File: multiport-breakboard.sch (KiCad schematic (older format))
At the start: 6 parts, among them J1 USB_terminal, J2 USB_B_Micro, J3 soldier_pads, J4 MULT_terminal, SW1 SW_SPDT_MSM

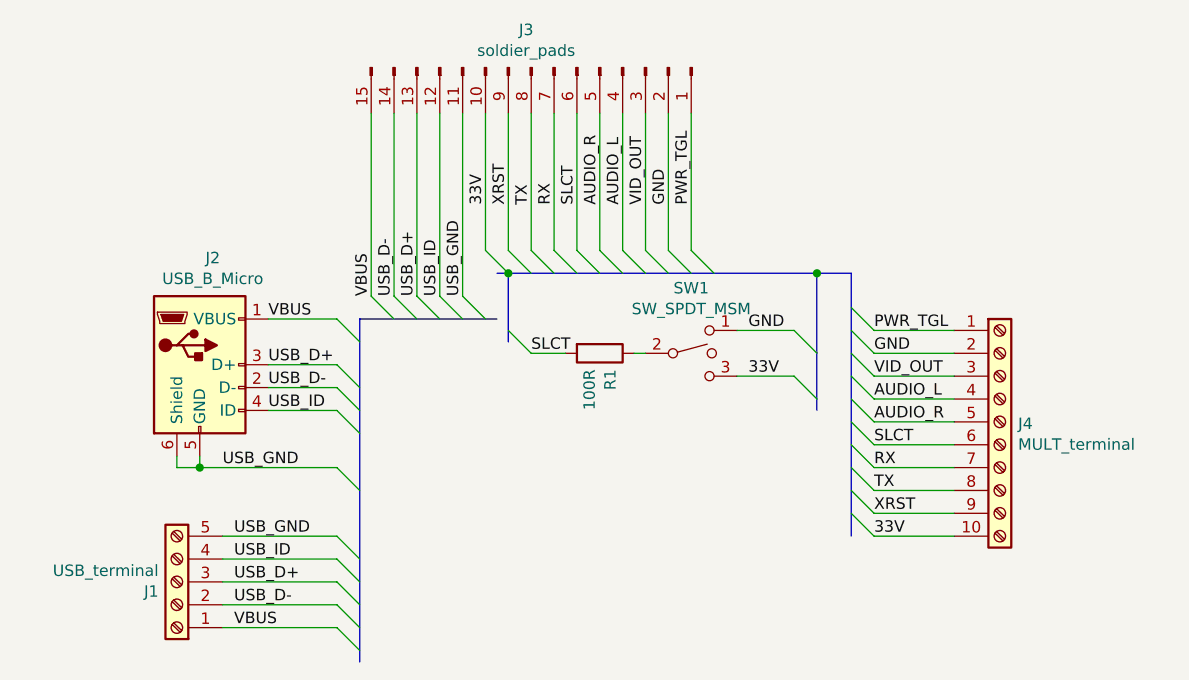
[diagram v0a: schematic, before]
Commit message: Revision 0.1
Revision just before submiting to david
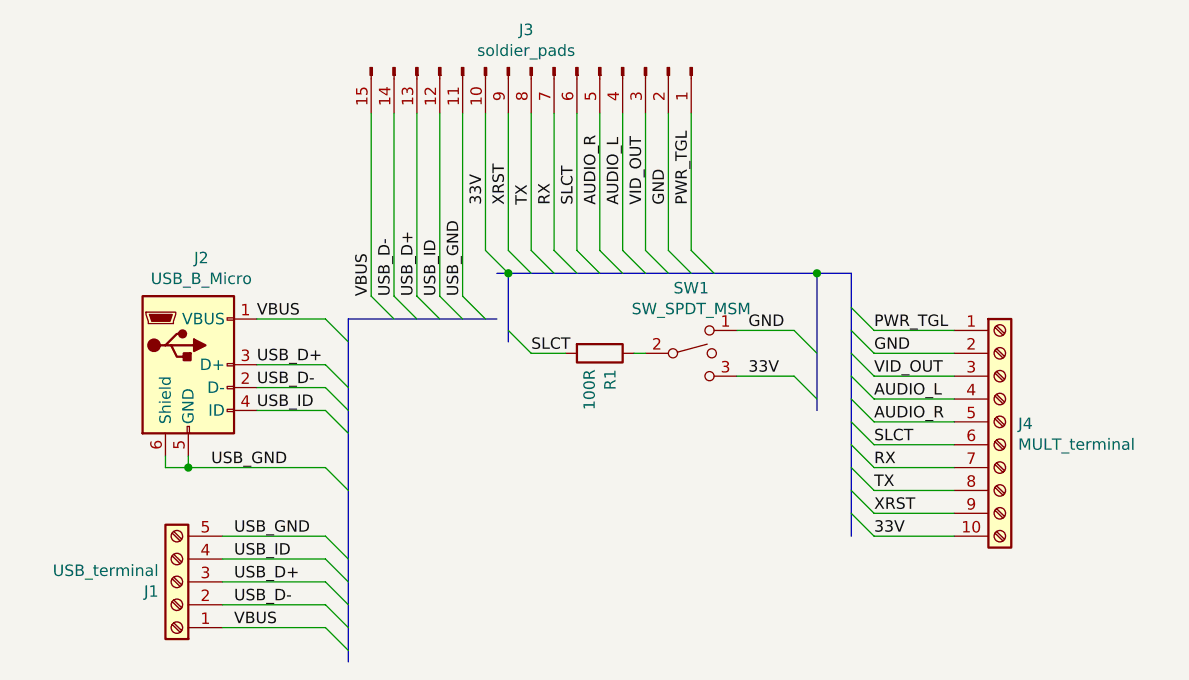
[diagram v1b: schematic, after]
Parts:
- J3: footprint Connector_Dsub:DSUB-15_Male_Horizontal_P2.77x2.84mm_EdgePinOffset9.40mm -> Connector_Dsub:DSUB-15_Female_Horizontal_P2.77x2.84mm_EdgePinOffset9.40mm
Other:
- moved on the sheet: J2
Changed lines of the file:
@@
 Text Label 1350 3200 0    50   ~ 0
 VBUS
-Connection ~ 1200 2500
-Wire Wire Line
-	1100 2500 1200 2500
-Wire Wire Line
-	1100 2450 1100 2500
-Text Label 1300 2500 0    50   ~ 0
-USB_GND
-Text Label 1500 2250 0    50   ~ 0
-USB_ID
-Text Label 1500 2150 0    50   ~ 0
-USB_D-
-Text Label 1500 2050 0    50   ~ 0
-USB_D+
-Text Label 1500 1850 0    50   ~ 0
-VBUS
 Text Label 2350 1750 1    50   ~ 0
 USB_GND
@@
 	-1   0    0    1
 $EndComp
-$Comp
-L Connector:USB_B_Micro J2
-U 1 1 5EC78F39
-P 1200 2050
-F 0 "J2" H 1257 2517 50  0000 C CNN
-F 1 "USB_B_Micro" H 1257 2426 50  0000 C CNN
-F 2 "Connector_USB:USB_Micro-B_Molex_47346-0001" H 1350 2000 50  0001 C CNN
-F 3 "~" H 1350 2000 50  0001 C CNN
-	1    1200 2050
-	1    0    0    -1
-$EndComp
 Entry Wire Line
 	2350 1750 2450 1850
@@
 	1950 1750 1950 950
 Entry Wire Line
-	1800 2050 1900 2150
+	1750 2050 1850 2150
 Entry Wire Line
-	1800 2150 1900 2250
+	1750 2150 1850 2250
 Entry Wire Line
-	1800 2250 1900 2350
+	1750 2250 1850 2350
 Entry Wire Line
-	1800 1850 1900 1950
-Wire Wire Line
-	1800 1850 1500 1850
-Wire Wire Line
-	1800 2050 1500 2050
-Wire Wire Line
-	1800 2150 1500 2150
-Wire Wire Line
-	1800 2250 1500 2250
+	1750 1850 1850 1950
 Entry Wire Line
-	1800 2500 1900 2600
-Wire Wire Line
-	1800 2500 1200 2500
-Wire Wire Line
-	1200 2500 1200 2450
+	1750 2500 1850 2600
 Entry Wire Line
-	1800 2800 1900 2900
+	1750 2800 1850 2900
 Entry Wire Line
-	1800 2900 1900 3000
+	1750 2900 1850 3000
 Entry Wire Line
-	1800 3000 1900 3100
+	1750 3000 1850 3100
 Entry Wire Line
-	1800 3100 1900 3200
+	1750 3100 1850 3200
 Entry Wire Line
-	1800 3200 1900 3300
+	1750 3200 1850 3300
 Wire Wire Line
-	1300 2800 1800 2800
+	1300 2800 1750 2800
 Wire Wire Line
-	1300 2900 1800 2900
+	1300 2900 1750 2900
 Wire Wire Line
-	1300 3000 1800 3000
+	1300 3000 1750 3000
 Wire Wire Line
-	1300 3100 1800 3100
+	1300 3100 1750 3100
 Wire Wire Line
-	1300 3200 1800 3200
+	1300 3200 1750 3200
 Text Label 1950 1750 1    50   ~ 0
 VBUS
@@
 F 0 "J3" V 2485 728 50  0000 C CNN
 F 1 "soldier_pads" V 2576 728 50  0000 C CNN
-F 2 "Connector_Dsub:DSUB-15_Male_Horizontal_P2.77x2.84mm_EdgePinOffset9.40mm" H 2650 750 50  0001 C CNN
+F 2 "Connector_Dsub:DSUB-15_Female_Horizontal_P2.77x2.84mm_EdgePinOffset9.40mm" H 2650 750 50  0001 C CNN
 F 3 "~" H 2650 750 50  0001 C CNN
 	1    2650 750
@@
 $EndBitmap
 Wire Bus Line
-	2550 1650 2550 1950
+	1850 1850 1850 3350
 Wire Bus Line
-	3900 1650 3900 2250
+	1850 1850 2500 1850
 Wire Bus Line
-	1900 1850 2500 1850
+	2550 1650 3900 1650
 Wire Bus Line
-	1900 1850 1900 3350
+	2550 1650 2550 1950
 Wire Bus Line
 	4050 1650 4050 2800
 Wire Bus Line
-	2550 1650 3900 1650
+	3900 1650 3900 2250
+Wire Wire Line
+	1150 2500 1150 2450
+Wire Wire Line
+	1750 2500 1150 2500
+Wire Wire Line
+	1750 2250 1450 2250
+Wire Wire Line
+	1750 2150 1450 2150
+Wire Wire Line
+	1750 2050 1450 2050
+Wire Wire Line
+	1750 1850 1450 1850
+$Comp
+L Connector:USB_B_Micro J2
+U 1 1 5EC78F39
+P 1150 2050
+F 0 "J2" H 1207 2517 50  0000 C CNN
+F 1 "USB_B_Micro" H 1207 2426 50  0000 C CNN
+F 2 "Connector_USB:USB_Micro-B_Molex_47346-0001" H 1300 2000 50  0001 C CNN
+F 3 "~" H 1300 2000 50  0001 C CNN
+	1    1150 2050
+	1    0    0    -1
+$EndComp
+Text Label 1450 1850 0    50   ~ 0
+VBUS
+Text Label 1450 2050 0    50   ~ 0
+USB_D+
+Text Label 1450 2150 0    50   ~ 0
+USB_D-
+Text Label 1450 2250 0    50   ~ 0
+USB_ID
+Text Label 1250 2500 0    50   ~ 0
+USB_GND
+Wire Wire Line
+	1050 2450 1050 2500
+Wire Wire Line
+	1050 2500 1150 2500
+Connection ~ 1150 2500
 $EndSCHEMATC
